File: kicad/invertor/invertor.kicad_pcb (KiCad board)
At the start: 2 copper layers, 24.6 x 14.7 mm, 23 parts, among them J1 Conn, J2 Conn, J3 Conn, J4 Conn, J5 Conn, J6 Conn, Q1 IRF7343PBF, Q2 IRF7343PBF, Q3 IRLML6344, Q4 IRLML6344

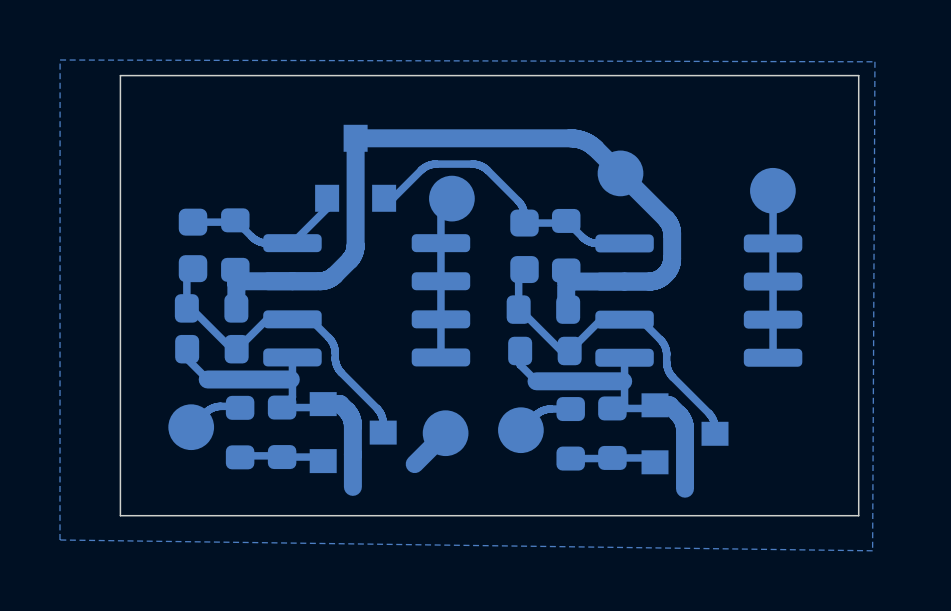
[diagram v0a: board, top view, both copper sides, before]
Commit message: изменено:      kicad/invertor/fp-info-cache 	изменено:      kicad/invertor/invertor.kicad_pcb
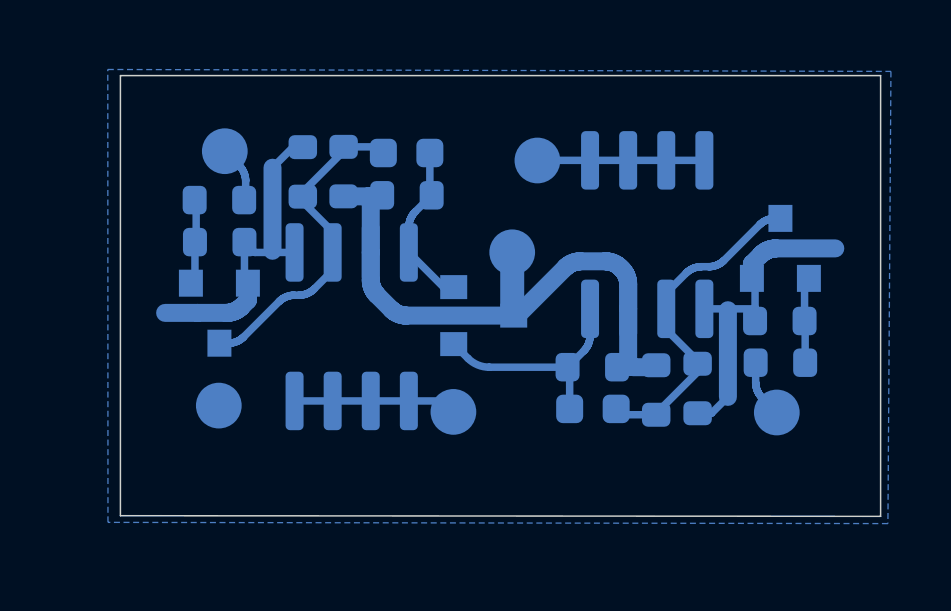
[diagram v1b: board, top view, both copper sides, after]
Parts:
- moved J3 9.27 mm to (33.9, 39.3), turned to -90 degrees
- moved J2 8.55 mm to (52.3, 48.0), turned to 90 degrees
- moved J5 7.91 mm to (44.4, 39.6), turned to 90 degrees
- moved R6 7.78 mm to (33.8, 40.9), turned to 0 degrees
- moved C1 7.76 mm to (40.0, 39.3), turned to 180 degrees
- moved J6 7.62 mm to (33.7, 47.8), turned to -90 degrees
- moved R9 7.38 mm to (52.5, 46.3), turned to 0 degrees
- moved J1 7.11 mm to (41.6, 48.0), turned to -90 degrees
- moved Q4 6.95 mm to (52.5, 42.5), turned to 90 degrees
- moved R5 6.72 mm to (52.4, 44.9), turned to 180 degrees
- moved R8 6.67 mm to (33.8, 42.3), turned to 0 degrees
- moved R2 6.64 mm to (36.5, 40.0), turned to 90 degrees
- moved D2 6.51 mm to (42.6, 44.8), turned to 0 degrees
- moved R7 6.34 mm to (37.9, 40.0), turned to 90 degrees
- moved Q3 5.98 mm to (33.8, 44.7), turned to -90 degrees
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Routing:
- net /+12v: track 27.6 -> 20.4 mm
- net Net-(C3-Pad1): track 9.82 -> 7.71 mm
- net GND: track 23.1 -> 21.6 mm
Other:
- board size 24.6 x 14.7 mm -> 25.3 x 14.7 mm
- net class Default removed
